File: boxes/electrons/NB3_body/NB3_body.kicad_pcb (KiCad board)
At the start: 2 copper layers, 200 x 199.5 mm, 21 parts, among them J1 Conn_01x02_Male, J2 Conn_01x02_Male, J3 Conn_01x02_Male, J4 Conn_01x02_Male, J5 Conn_01x04_Male, J6 Conn_01x02_Male

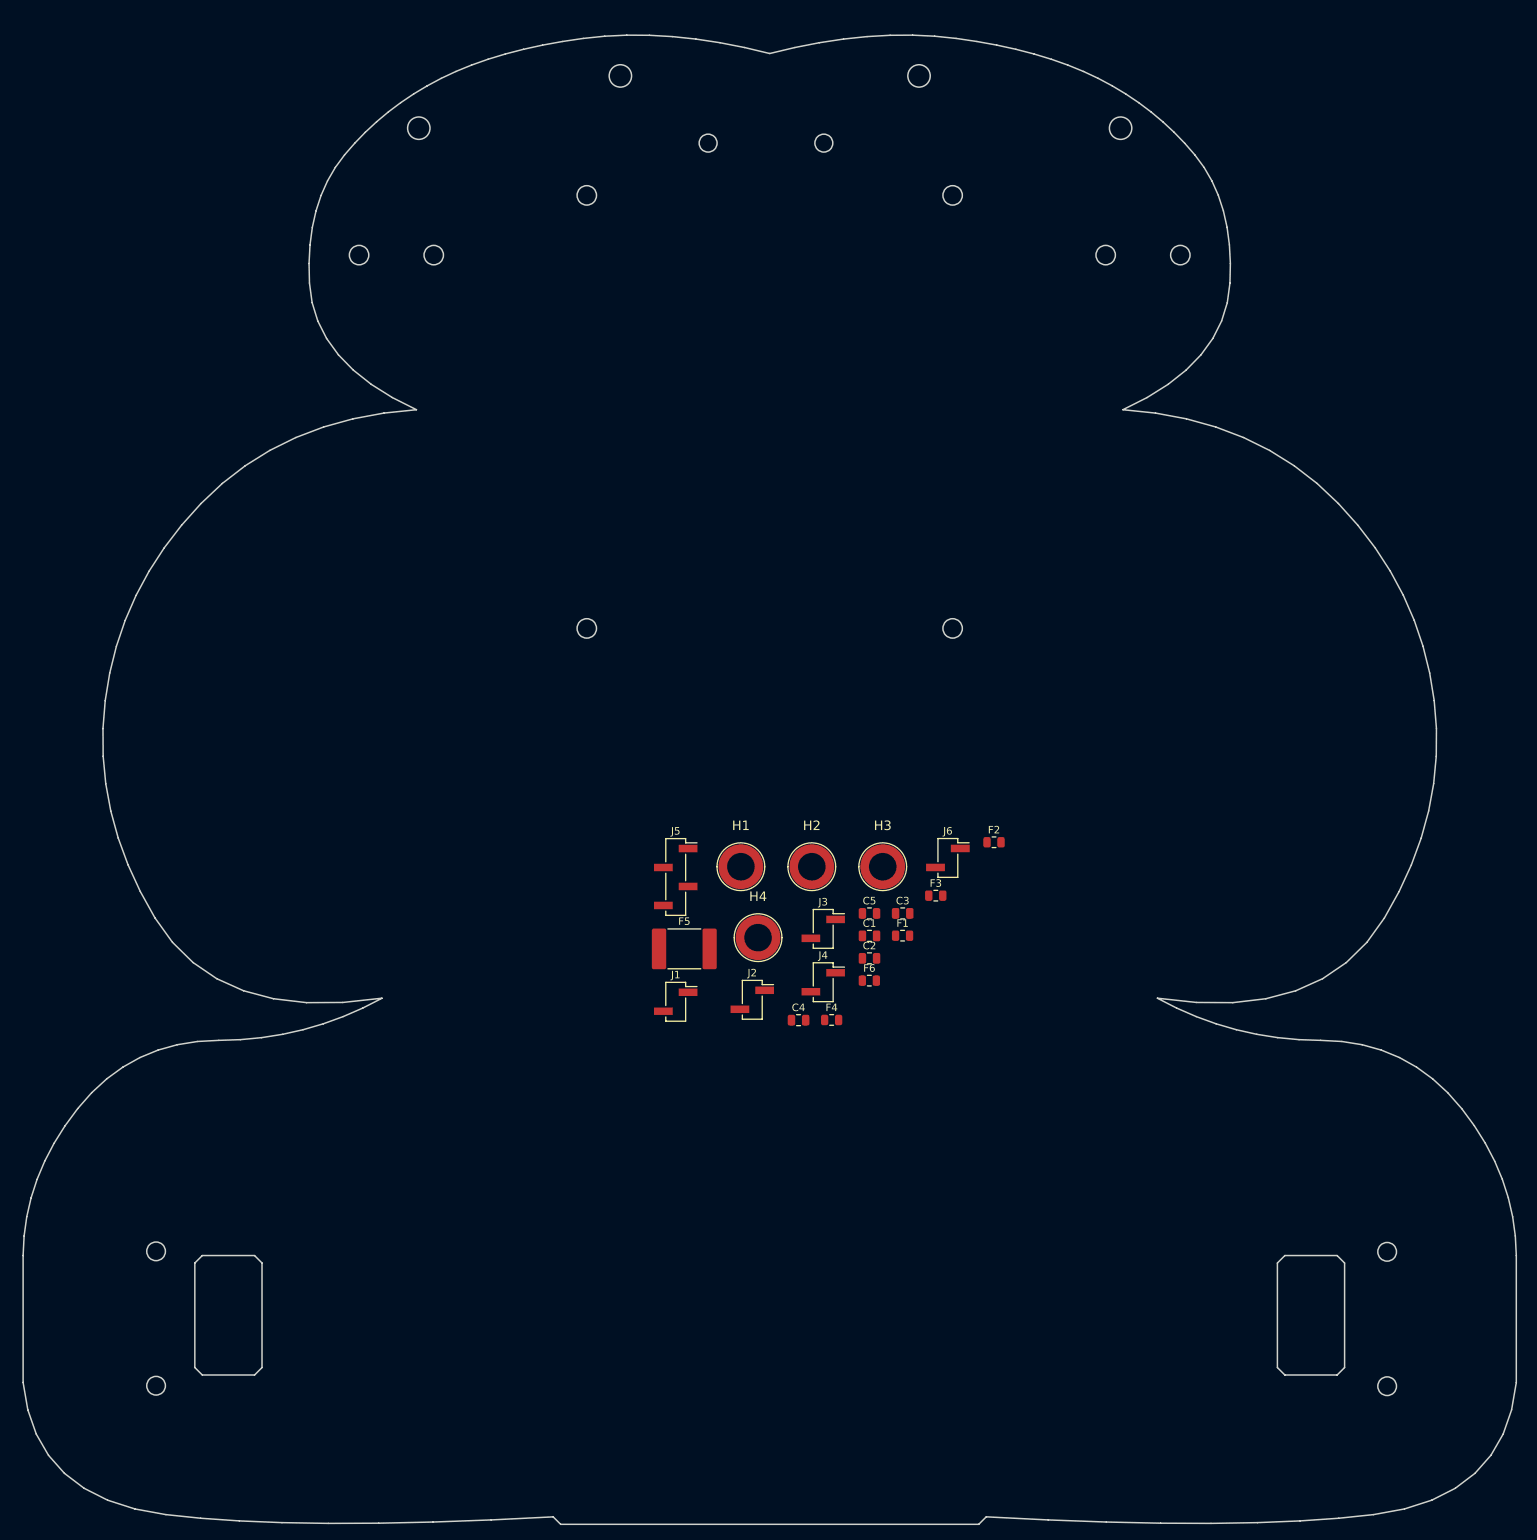
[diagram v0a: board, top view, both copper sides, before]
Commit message: Work on NB3_body PCB...
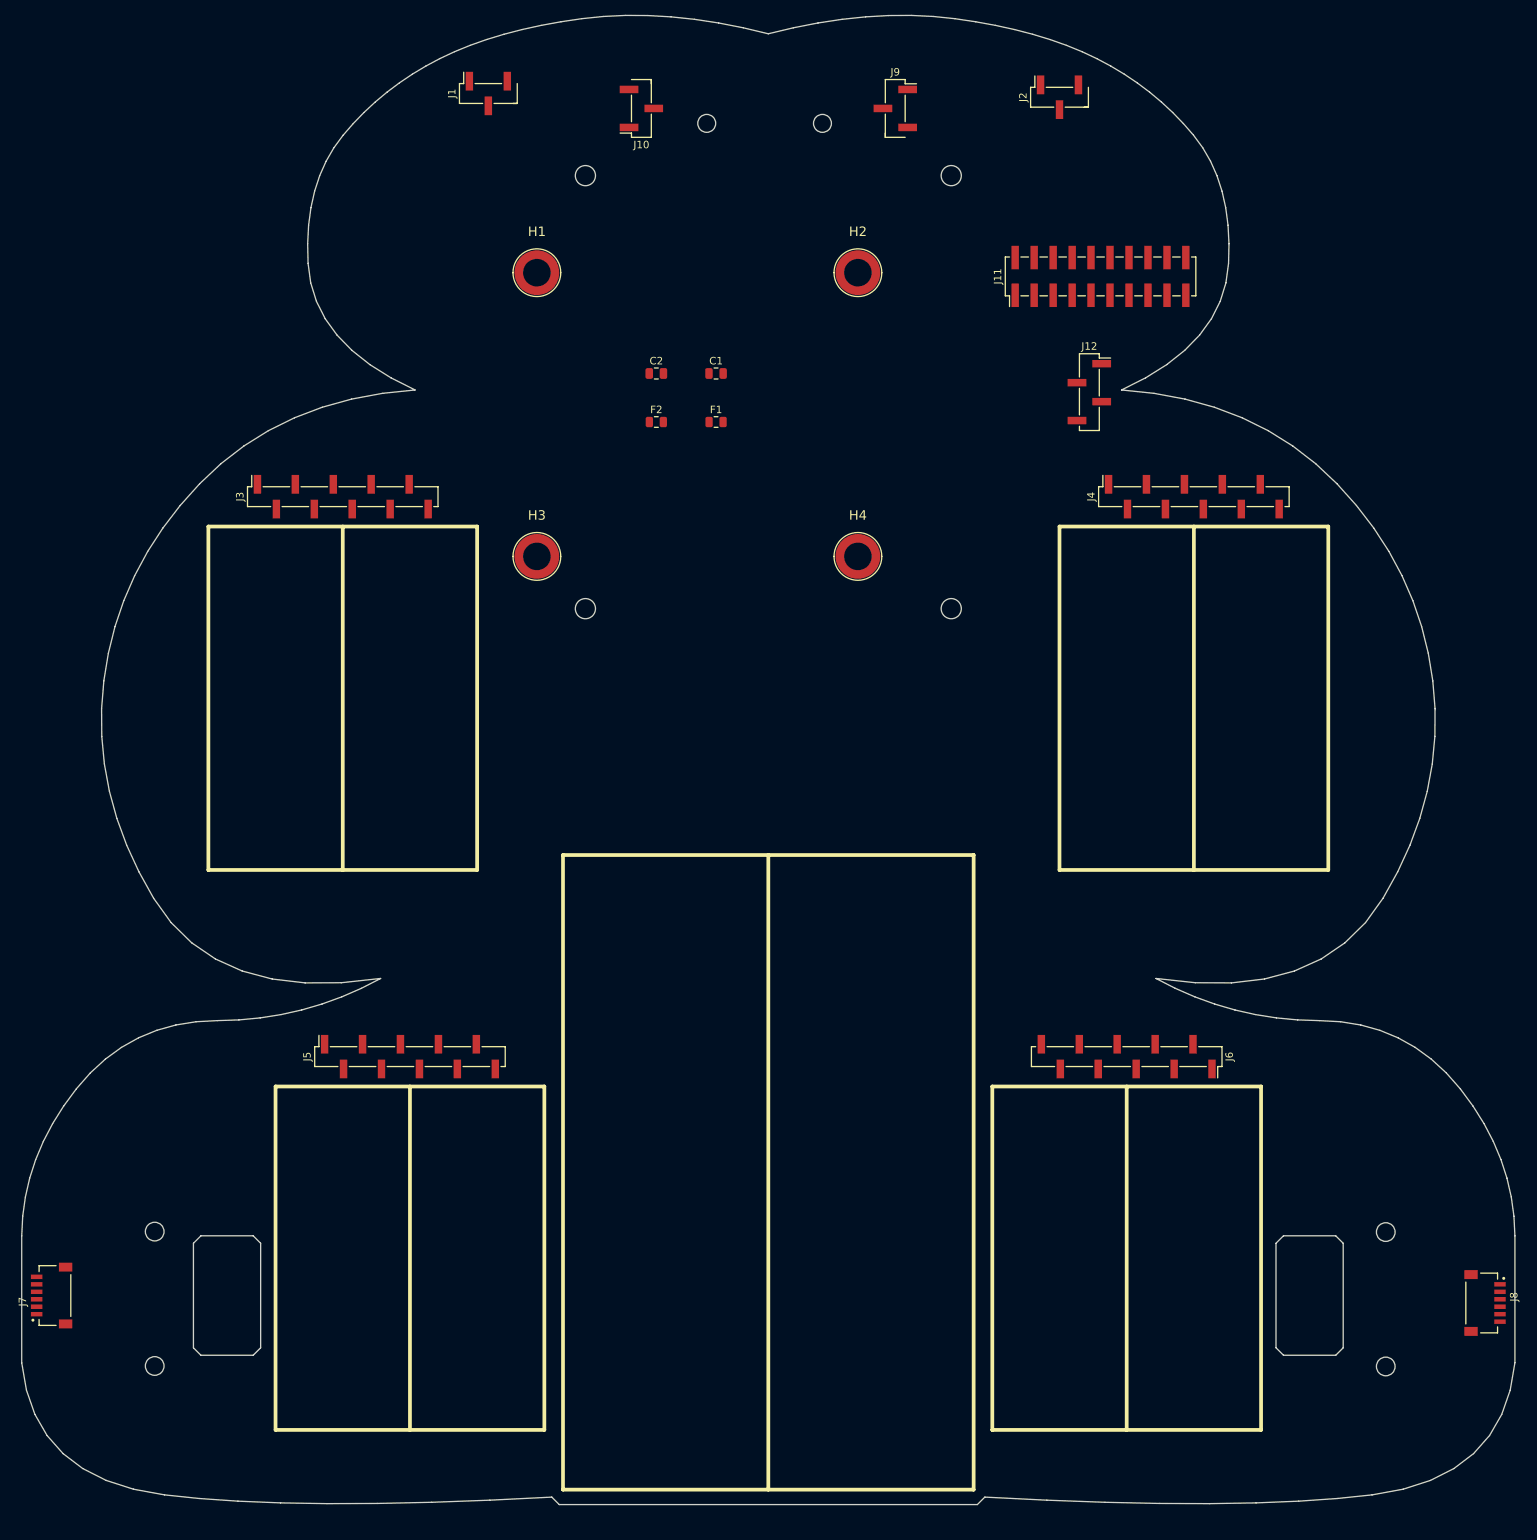
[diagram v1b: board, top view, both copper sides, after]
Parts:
- removed C3, C4, C5: 10uF, Capacitor_SMD:C_0805_2012Metric
- removed F3, F4, F6: 1.1h2.2t, Fuse:Fuse_0805_2012Metric
- removed F5: 3h5t, Fuse:Fuse_2920_7451Metric
- added J10: Conn_01x03_Female, Connector_PinHeader_2.54mm:PinHeader_1x03_P2.54mm_Vertical_SMD_Pin1Right, F.Cu at (107.5, 36.0)
- added J11: Conn_02x10_Odd_Even, Connector_PinHeader_2.54mm:PinHeader_2x10_P2.54mm_Vertical_SMD, F.Cu at (169.0, 58.5)
- added J12: Conn_01x04_Male, Connector_PinHeader_2.54mm:PinHeader_1x04_P2.54mm_Vertical_SMD_Pin1Right, F.Cu at (167.5, 74.0)
- added J7: Socket_SM06B-SRSS-TB, NB3_body:Socket_SM06B-SRSS-TB, F.Cu at (26.5, 195.0)
- added J8: Socket_SM06B-SRSS-TB, NB3_body:Socket_SM06B-SRSS-TB, F.Cu at (222.5, 196.0)
- added J9: Conn_01x03_Female, Connector_PinHeader_2.54mm:PinHeader_1x03_P2.54mm_Vertical_SMD_Pin1Right, F.Cu at (141.5, 36.0)
- J1, J2: value Conn_01x02_Male -> Conn_01x03_Female; footprint Connector_PinHeader_2.54mm:PinHeader_1x02_P2.54mm_Vertical_SMD_Pin1Right -> Connector_PinHeader_2.54mm:PinHeader_1x03_P2.54mm_Vertical_SMD_Pin1Right
- J3, J4, J6: value Conn_01x02_Male -> Conn_01x10_Male; footprint Connector_PinHeader_2.54mm:PinHeader_1x02_P2.54mm_Vertical_SMD_Pin1Right -> Connector_PinHeader_2.54mm:PinHeader_1x10_P2.54mm_Vertical_SMD_Pin1Right
- J5: value Conn_01x04_Male -> Conn_01x10_Male; footprint Connector_PinHeader_2.54mm:PinHeader_1x04_P2.54mm_Vertical_SMD_Pin1Right -> Connector_PinHeader_2.54mm:PinHeader_1x10_P2.54mm_Vertical_SMD_Pin1Right
- moved J2 127.7 mm to (163.5, 34.5), turned to 90 degrees
- moved J1 124.2 mm to (87.0, 34.0), turned to 90 degrees
- moved J3 86.6 mm to (67.5, 88.0), turned to 90 degrees
- moved H1 84.1 mm to (93.5, 58.0)
- moved C2 83.4 mm to (109.5, 71.5)
- moved J4 81.8 mm to (181.5, 88.0), turned to 90 degrees
- moved H2 79.8 mm to (136.5, 58.0)
- moved C1 78.1 mm to (117.5, 71.5)
- moved F1 73.2 mm to (117.5, 78.0)
- moved F2 72.2 mm to (109.5, 78.0)
- moved H3 62.2 mm to (93.5, 96.0)
- moved H4 52.8 mm to (136.5, 96.0)
- moved J5 43.0 mm to (76.5, 163.0), turned to 90 degrees
- moved J6 35.8 mm to (172.5, 163.0), turned to -90 degrees
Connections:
- C1 pad 1: +5V -> unconnected-(C1-Pad1)
- C1 pad 2: GND -> unconnected-(C1-Pad2)
- C2 pad 1: +5V -> unconnected-(C2-Pad1)
- C2 pad 2: GND -> unconnected-(C2-Pad2)
- F1 pad 1: Net-(F1-Pad1) -> unconnected-(F1-Pad1)
- F1 pad 2: +5V -> unconnected-(F1-Pad2)
- F2 pad 1: Net-(F2-Pad1) -> unconnected-(F2-Pad1)
- F2 pad 2: +5V -> unconnected-(F2-Pad2)
- J1 pad 1: GND -> unconnected-(J1-Pad1)
- J1 pad 2: Net-(F1-Pad1) -> unconnected-(J1-Pad2)
- J2 pad 1: GND -> unconnected-(J2-Pad1)
- J2 pad 2: Net-(F2-Pad1) -> unconnected-(J2-Pad2)
- J3 pad 1: GND -> unconnected-(J3-Pad1)
- J3 pad 2: Net-(F3-Pad1) -> unconnected-(J3-Pad2)
- J4 pad 1: GND -> unconnected-(J4-Pad1)
- J4 pad 2: Net-(F4-Pad1) -> unconnected-(J4-Pad2)
- J5 pad 1: GND -> unconnected-(J5-Pad1)
- J5 pad 2: GND -> unconnected-(J5-Pad2)
- J5 pad 3: Net-(F5-Pad1) -> unconnected-(J5-Pad3)
- J5 pad 4: Net-(F5-Pad1) -> unconnected-(J5-Pad4)
- J6 pad 1: GND -> unconnected-(J6-Pad1)
- J6 pad 2: Net-(F6-Pad1) -> unconnected-(J6-Pad2)
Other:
- outline, holes or cut-outs redrawn
